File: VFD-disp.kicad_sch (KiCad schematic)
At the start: 97 parts, among them J1 USB_C_Receptacle_USB2.0_14P, J2 Conn_02x04_Odd_Even, J3 Jack-DC, J4 Conn_02x04_Odd_Even, J5 Conn_02x04_Odd_Even, J6 Conn_02x04_Odd_Even, Q1 NMOS, Q3 NMOS, SW1 SW_SPST, U1 ESP32-C6-WROOM-1, U10 TXS0104EPW, U11 MAX811TEUS-T, U12 MCP4728, U2 FUSB302B01MPX, U3 LM1117DT-3.3, U4 MCP1416, U5 LM2576HVS-ADJ, U6 MAX1771xSA, U7 LM2576HVS-ADJ, U9 FM24C64B, Y1 Crystal

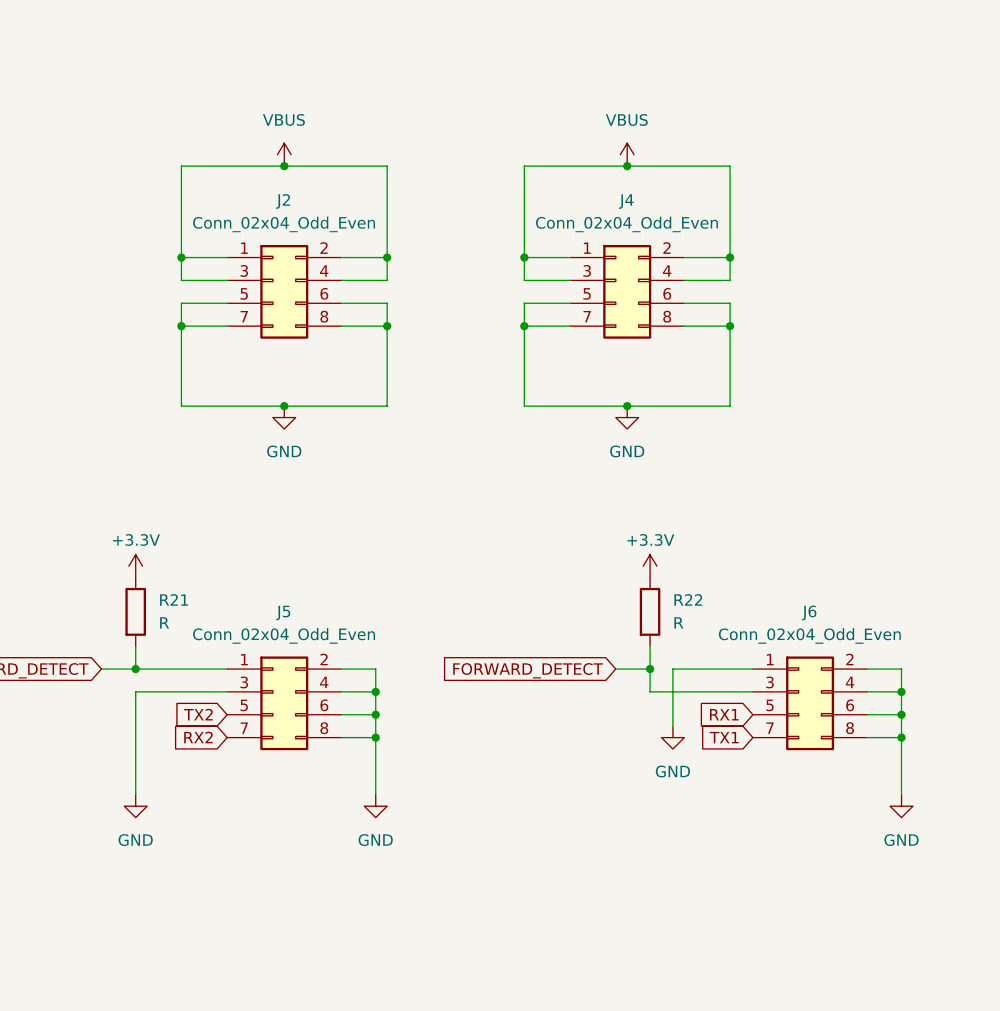
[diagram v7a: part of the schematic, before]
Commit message: We need to golf!
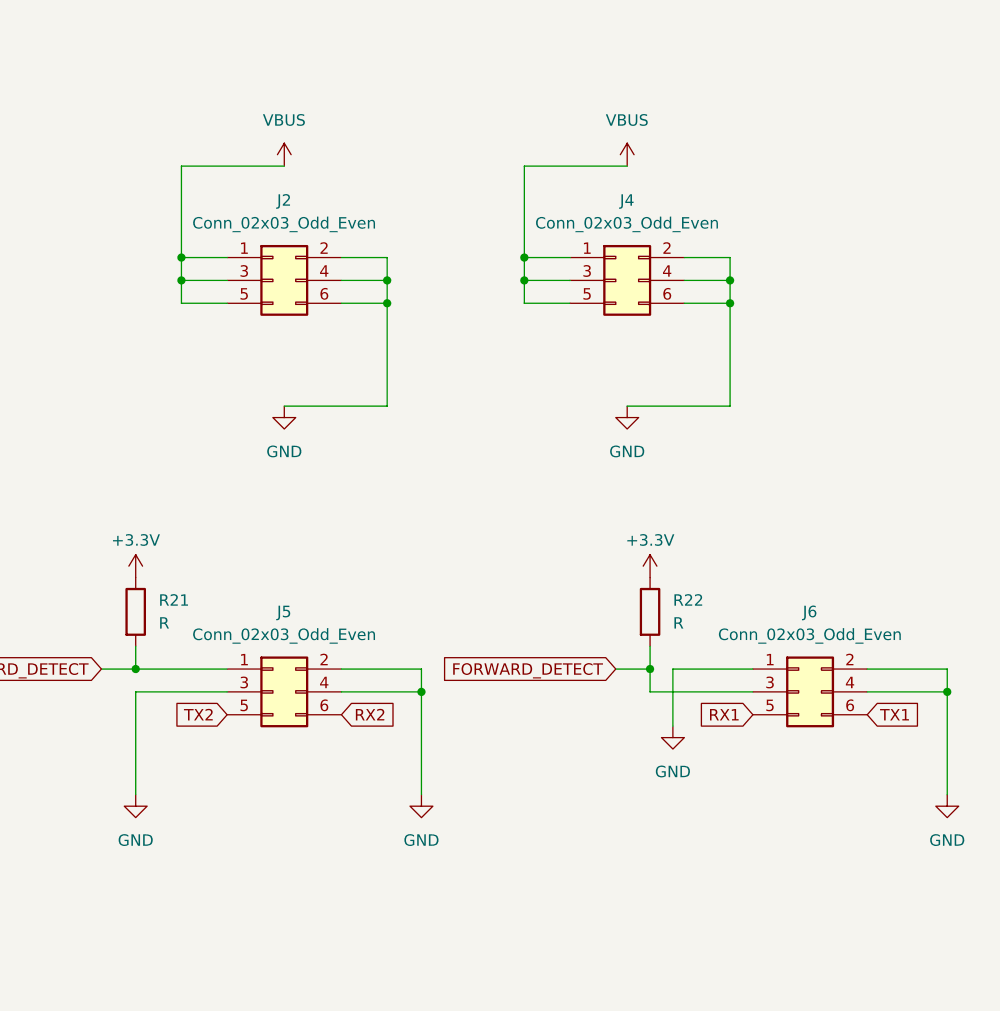
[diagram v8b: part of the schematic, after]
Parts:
- J2, J5: value Conn_02x04_Odd_Even -> Conn_02x03_Odd_Even; footprint Connector_PinSocket_2.54mm:PinSocket_2x04_P2.54mm_Horizontal -> Connector_PinSocket_2.54mm:PinSocket_2x03_P2.54mm_Horizontal; symbol Connector_Generic:Conn_02x04_Odd_Even -> Connector_Generic:Conn_02x03_Odd_Even
- J4, J6: value Conn_02x04_Odd_Even -> Conn_02x03_Odd_Even; footprint Connector_PinHeader_2.54mm:PinHeader_2x04_P2.54mm_Horizontal -> Connector_PinHeader_2.54mm:PinHeader_2x03_P2.54mm_Horizontal; symbol Connector_Generic:Conn_02x04_Odd_Even -> Connector_Generic:Conn_02x03_Odd_Even
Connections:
- net GND: now also J2.2 (Pin_2), J2.4 (Pin_4), J4.2 (Pin_2), J4.4 (Pin_4); no longer J2.5 (Pin_5), J2.7 (Pin_7), J2.8 (Pin_8), J4.5 (Pin_5), J4.7 (Pin_7), J4.8 (Pin_8), J5.6 (Pin_6), J5.8 (Pin_8), J6.6 (Pin_6), J6.8 (Pin_8)
- net RX2: now also J5.6 (Pin_6); no longer J5.7 (Pin_7)
- net TX1: now also J6.6 (Pin_6); no longer J6.7 (Pin_7)
- net VBUS: now also J2.5 (Pin_5), J4.5 (Pin_5); no longer J2.2 (Pin_2), J2.4 (Pin_4), J4.2 (Pin_2), J4.4 (Pin_4)
